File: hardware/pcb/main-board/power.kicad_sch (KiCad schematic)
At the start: 20 parts, among them Q501 DMG2302U, SW501 NO POP, SW502 NO POP, U501 PT4110, U502 AZ1117H-3.3_SOT223

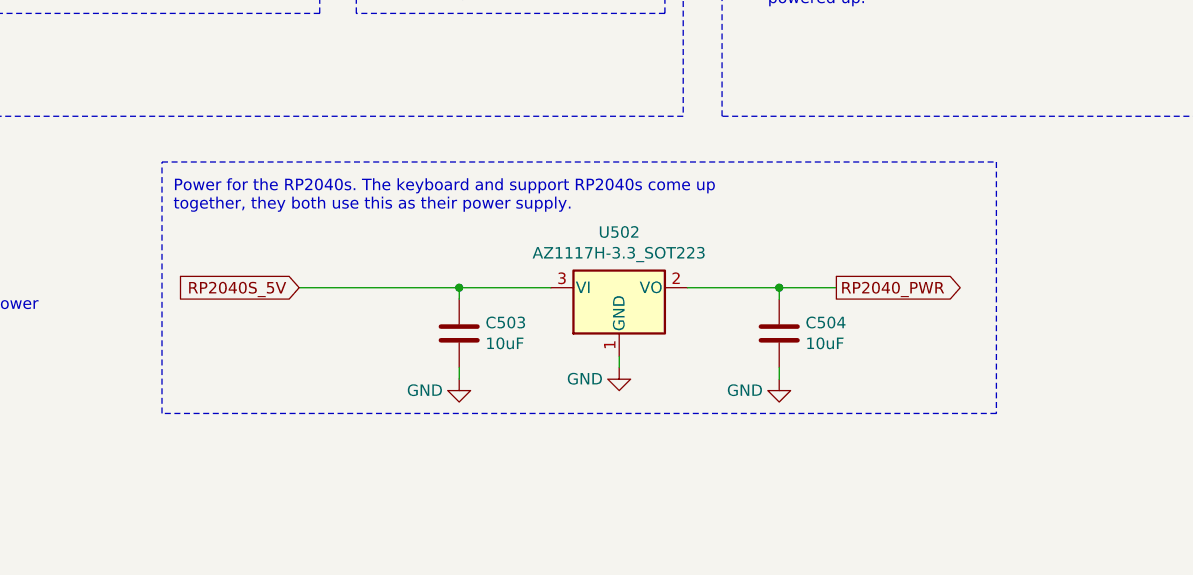
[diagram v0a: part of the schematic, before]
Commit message: a few more tidyups, almost ready for dual shifts stuff now
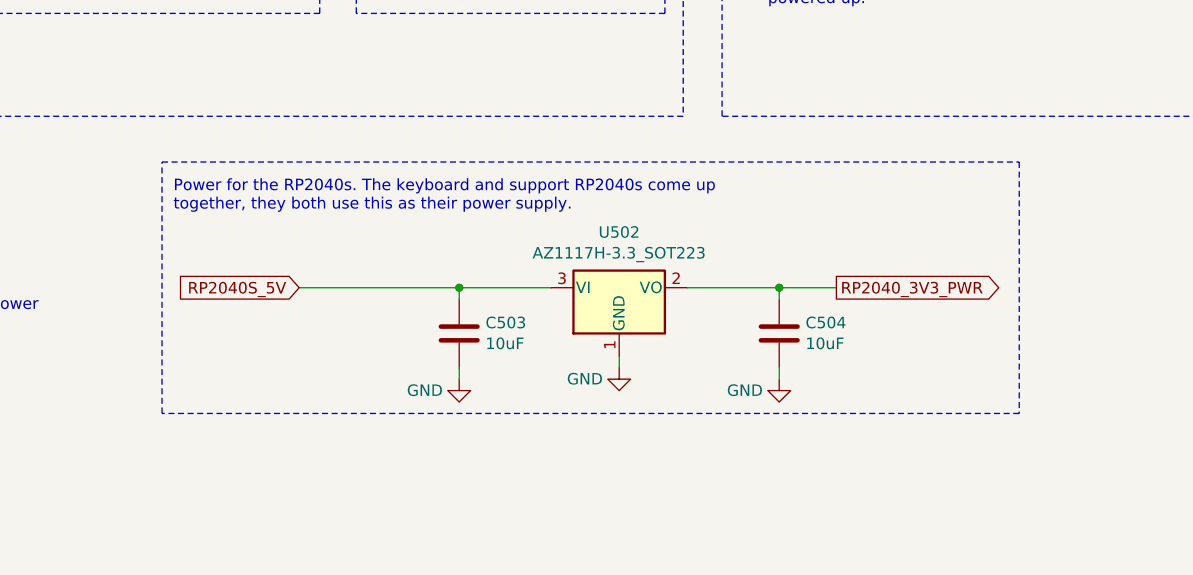
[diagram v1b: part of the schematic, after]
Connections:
- net RP2040_PWR renamed RP2040_3V3_PWR
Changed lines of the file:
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@@
 	(rectangle
 		(start 83.82 72.39)
-		(end 176.53 100.33)
+		(end 179.07 100.33)
 		(stroke
 			(width 0)
@@
 		)
 	)
-	(global_label "RP2040_PWR"
+	(global_label "RP2040_3V3_PWR"
 		(shape output)
 		(at 158.75 86.36 0)
